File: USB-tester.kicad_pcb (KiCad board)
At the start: 2 copper layers, 68.7 x 41.2 mm, 57 parts

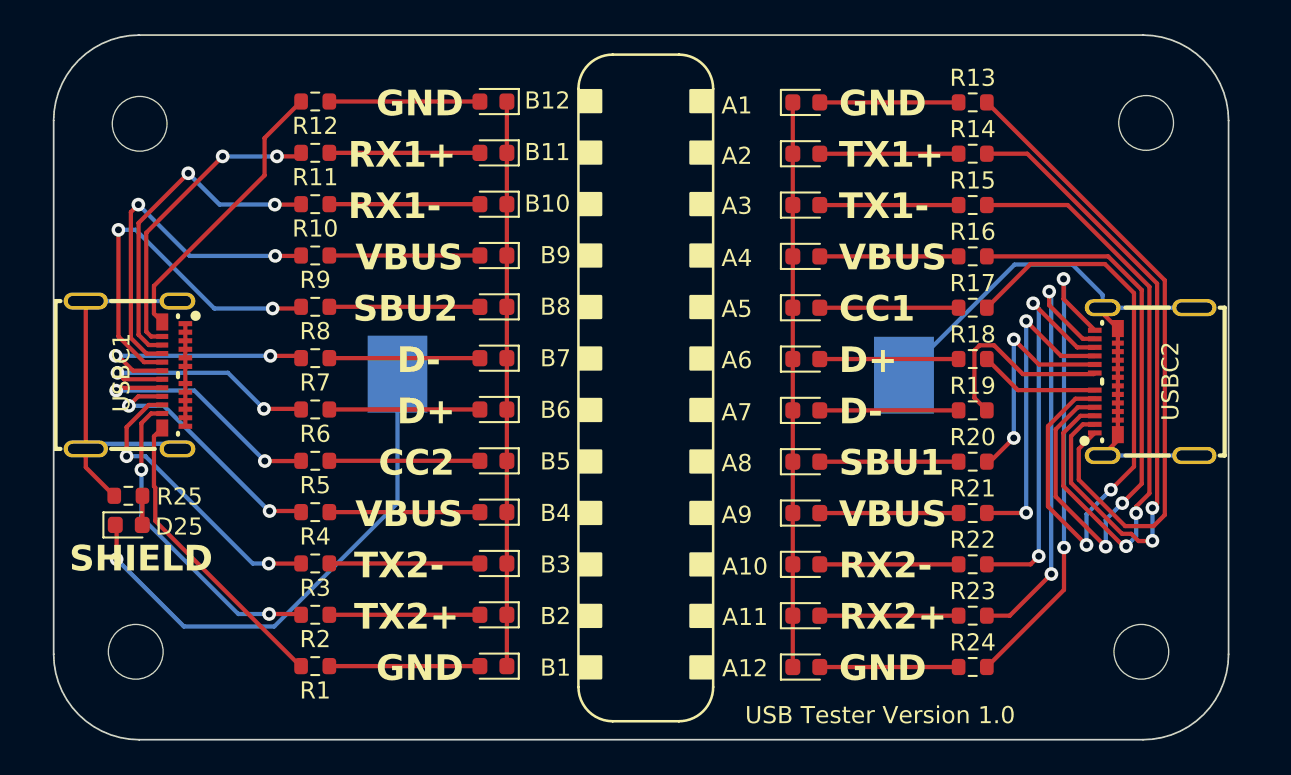
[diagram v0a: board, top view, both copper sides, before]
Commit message: Version 2
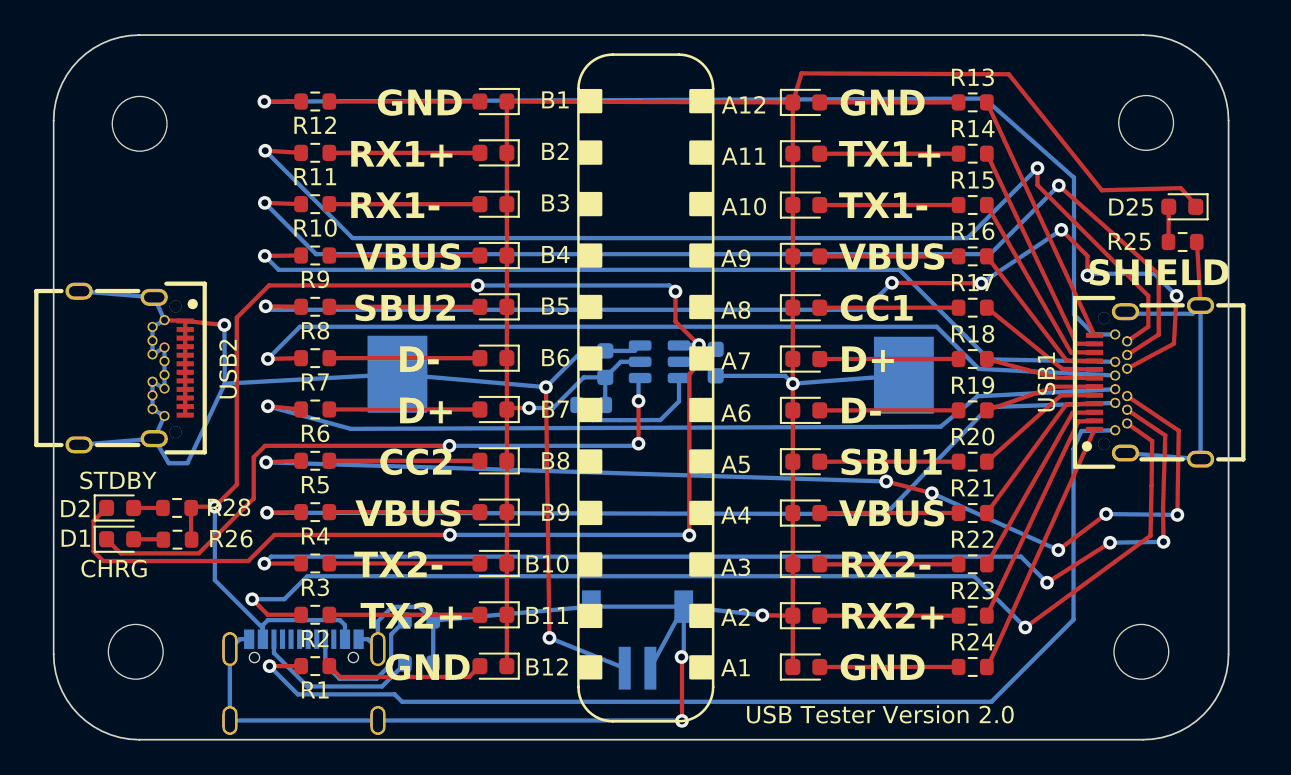
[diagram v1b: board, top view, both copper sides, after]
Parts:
- removed USBC1, USBC2: 105450-0101, USB-C-SMD_TYPE-C-USB-18:USB-C-SMD_TYPE-C-USB-18
- added BAT1: S2B-ZR-SM4A-TF_LF__SN_, S2B-ZR-SM4A-TF_LF__SN_:JST_S2B-ZR-SM4A-TF_LF__SN_, B.Cu at (166.4, 116.1)
- added C1: 10uF, Capacitor_SMD:C_0603_1608Metric, B.Cu at (164.5, 100.5)
- added C2: 10uF, Capacitor_SMD:C_0603_1608Metric, B.Cu at (171.0, 100.4)
- added D1: RED, LED_SMD:LED_0603_1608Metric, F.Cu at (136.1, 110.7)
- added D2: GREEN, LED_SMD:LED_0603_1608Metric, F.Cu at (136.1, 108.9)
- added J1: TYPE-C-31-M-12, TYPE-C-31-M-12:HRO_TYPE-C-31-M-12, B.Cu at (146.9, 121.3)
- added R26: 220R, Resistor_SMD:R_0603_1608Metric, F.Cu at (139.5, 110.7)
- added R27: 5.1K, Resistor_SMD:R_0603_1608Metric, B.Cu at (163.7, 102.8)
- added R28: 220R, Resistor_SMD:R_0603_1608Metric, F.Cu at (139.5, 108.9)
- added R29: 5.1K, Resistor_SMD:R_0603_1608Metric, B.Cu at (153.6, 115.4)
- added R30: 5.1K, Resistor_SMD:R_0603_1608Metric, B.Cu at (153.6, 118.0)
- added U1: TP4057, Package_TO_SOT_SMD:SOT-23-6, B.Cu at (167.7, 100.3)
- added USB1: TYPEC-324-BCP24, easyeda2kicad:USB-C-SMD_TYPEC-324-BCP24, F.Cu at (196.2, 101.5)
- added USB2: TYPEC-324-BCP24, easyeda2kicad:USB-C-SMD_TYPEC-324-BCP24, F.Cu at (136.8, 100.7)
- moved D25 64.3 mm to (198.2, 91.3), turned to 180 degrees
- moved R25 63.4 mm to (198.2, 93.3), turned to 0 degrees
- turned BT2 to 0 degrees
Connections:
- net Net-(A1-K) renamed BAT-
- BT2 pad 1: A10_A -> A10_B
- R1 pad 2: B1_A -> B12_A
- R10 pad 2: B10_A -> B3_A
- R11 pad 2: B11_A -> B2_A
- R12 pad 2: B12_A -> B1_A
- R13 pad 2: A1_B -> A12_A
- R14 pad 2: A2_B -> A11_A
- R15 pad 2: A3_B -> A10_A
- R16 pad 2: A4_B -> A9_A
- R17 pad 2: A5_B -> A8_A
- R18 pad 2: A6_B -> A7_A
- R19 pad 2: A7_B -> A6_A
- R2 pad 2: B2_A -> B11_A
- R20 pad 2: A8_B -> A5_A
- R21 pad 2: A9_B -> A4_A
- R22 pad 2: A10_B -> A3_A
- R23 pad 2: A11_B -> A2_A
- R24 pad 2: A12_B -> A1_A
- R3 pad 2: B3_A -> B10_A
- R4 pad 2: B4_A -> B9_A
- R5 pad 2: B5_A -> B8_A
- R6 pad 2: B6_A -> B7_A
- R7 pad 2: B7_A -> B6_A
- R8 pad 2: B8_A -> B5_A
- R9 pad 2: B9_A -> B4_A
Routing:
- net BAT-: track 96.6 -> 206.7 mm, vias 1 -> 5
- net +5V: track 0.00 -> 63.0 mm, vias 0 -> 4
- net A10_B: track 22.8 -> 85.6 mm, vias 2 -> 3
- net Net-(D2-K): track 0.00 -> 50.2 mm, vias 0 -> 3
- net B5_A: track 15.3 -> 65.2 mm, vias 2 -> 6
- net B11_A: track 17.8 -> 66.6 mm
- net B12_A: track 16.6 -> 64.8 mm, vias 0 -> 1
- net B3_A: track 17.1 -> 65.0 mm
- net B2_A: track 18.6 -> 64.5 mm
- net B10_A: track 19.6 -> 65.1 mm, vias 2 -> 4
- net B1_A: track 17.7 -> 62.1 mm, vias 0 -> 1
- net B8_A: track 22.0 -> 65.4 mm, vias 2 -> 6
- net B4_A: track 14.8 -> 54.3 mm, vias 2 -> 1
- net Net-(D1-K): track 0.00 -> 39.4 mm, vias 0 -> 3
- net B6_A: track 14.4 -> 53.3 mm, vias 2 -> 1
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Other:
- board text added: "+"
- board text added: "-"
- board text added: "CHRG"
- board text added: "STDBY"
- board text added: "USB Tester Version 2.0"
- board text removed: "USB Tester Version 1.0"
